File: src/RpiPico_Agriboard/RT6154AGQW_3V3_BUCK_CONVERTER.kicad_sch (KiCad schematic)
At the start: 14 parts, among them U1 RT6154A/B

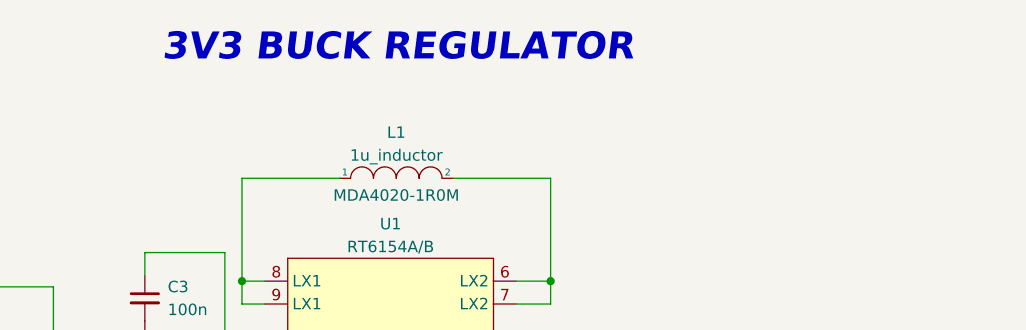
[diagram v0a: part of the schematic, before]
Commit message: schematic updates completed
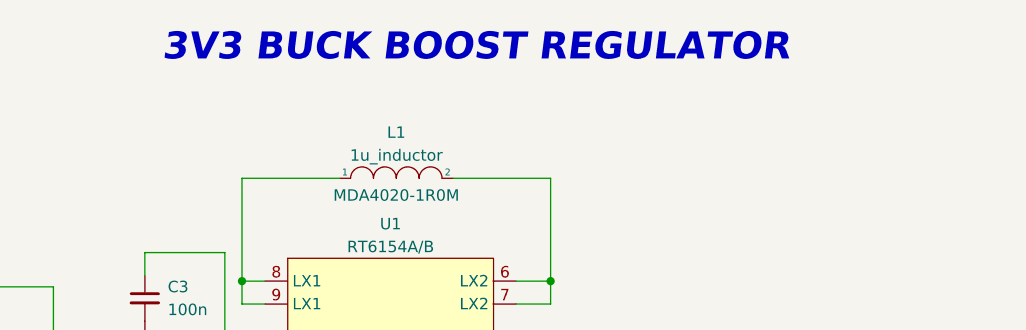
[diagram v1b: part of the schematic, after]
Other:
- note added: "3V3 BUCK BOOST REGULATOR"
- note removed: "3V3 BUCK REGULATOR"
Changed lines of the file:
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@@
     (stroke (width 0) (type default))
   )
-  (text "3V3 BUCK REGULATOR" (at 137.16 50.8 0)
+  (text "3V3 BUCK BOOST REGULATOR" (at 137.16 50.8 0)
     (effects (font (size 3 3) bold italic) (justify left bottom))
   )
